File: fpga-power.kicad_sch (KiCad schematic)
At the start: 81 parts, among them U15 XC7K160T-FFG676

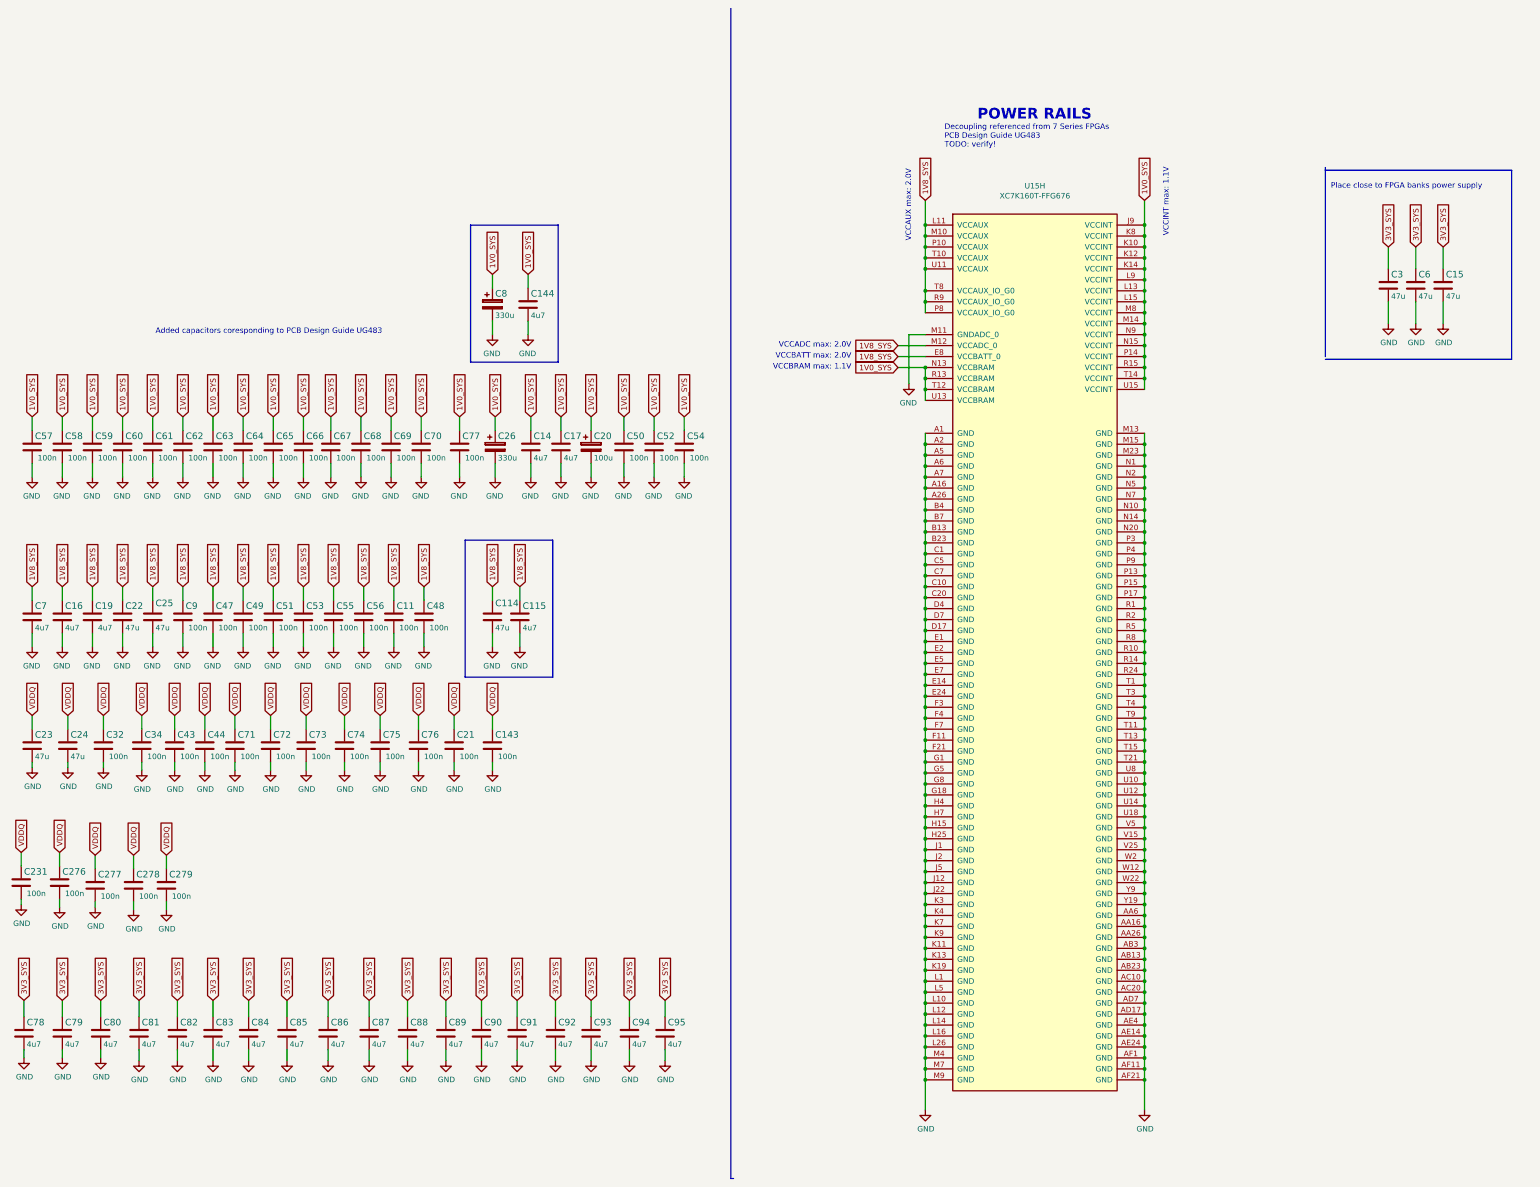
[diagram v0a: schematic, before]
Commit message: Cleanup schematic
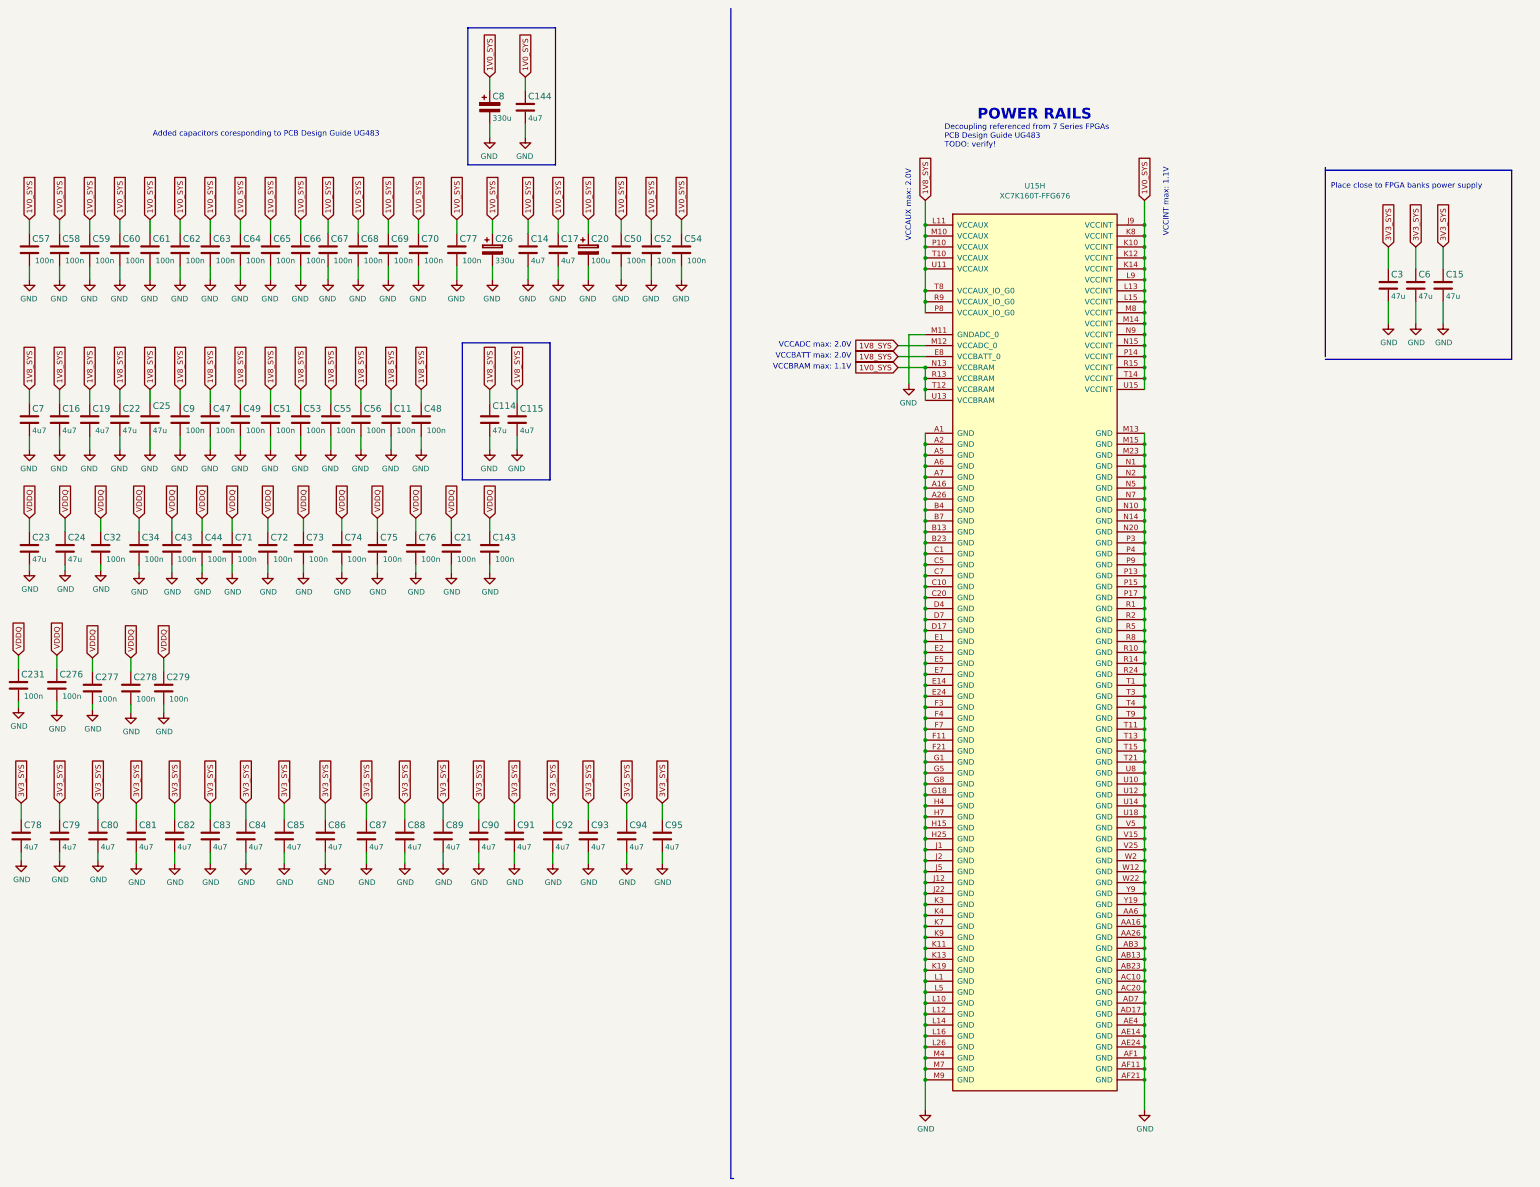
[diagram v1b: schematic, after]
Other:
- moved on the sheet: C11, C114, C115, C14, C143, C144, C16, C17, C19, C20, C21, C22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
